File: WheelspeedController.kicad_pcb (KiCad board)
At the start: 4 copper layers, 63.5 x 35.6 mm, 70 parts, among them J1 DEUTSCH DT Inp, J2 DEUTSCH DT Data, J3 DEUTSCH DT Out, J4 Conn_01x02, J6 SWD, SW1 SW_SPDT, SW2 SW_SPDT, U1 LMR51420, U2 AMS1117-3.3, U3 STM32F105RCTx, U4 SN65HVD230, Y1 16MHz

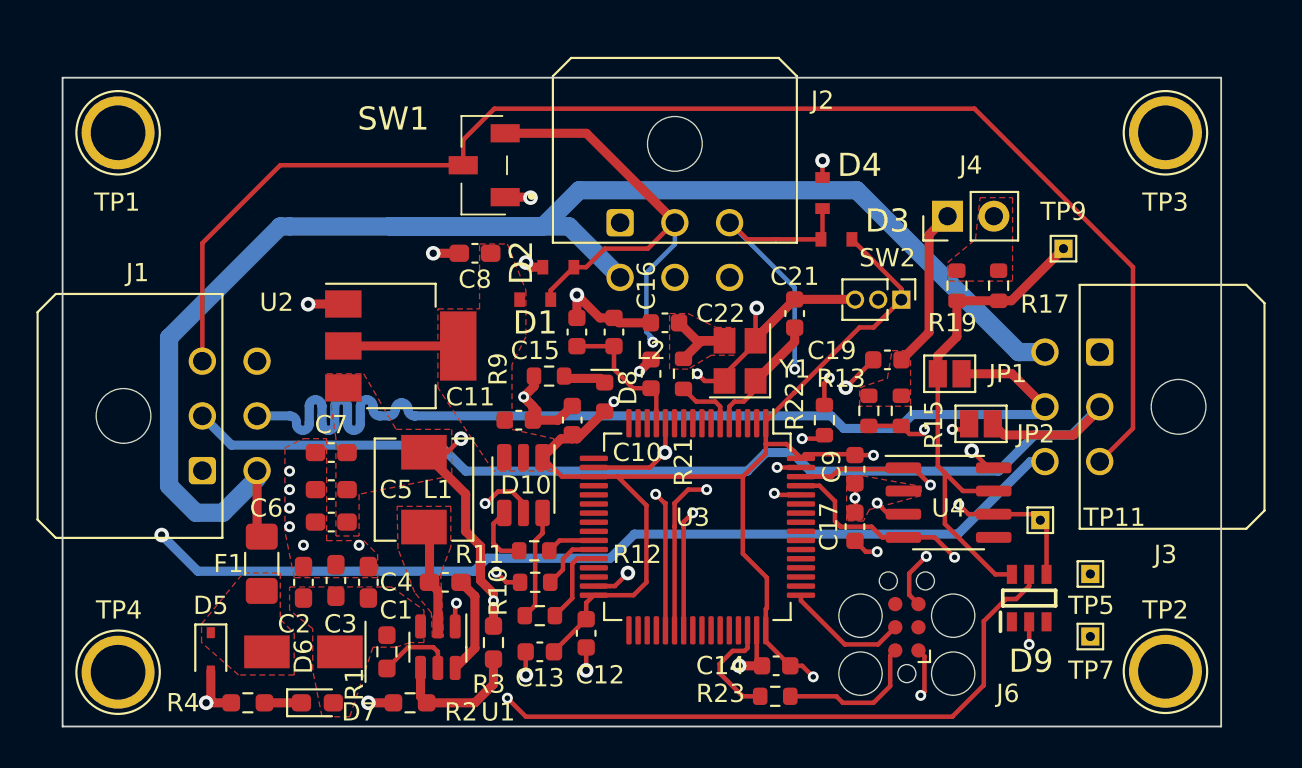
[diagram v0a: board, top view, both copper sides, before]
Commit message: Aligned connectors
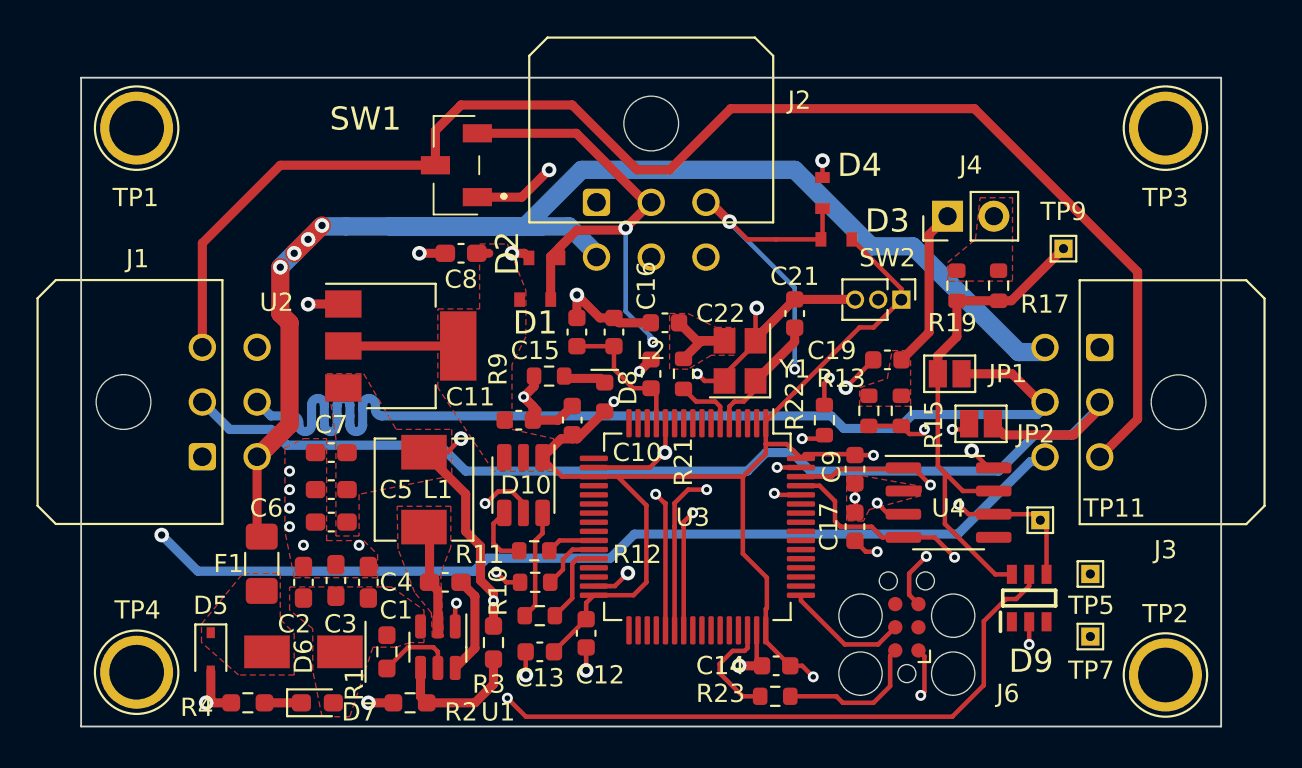
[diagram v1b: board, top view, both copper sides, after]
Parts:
- moved J2 1.71 mm to (87.2, 76.7)
- moved SW1 1.52 mm to (79.5, 74.7)
- moved TP1 1.05 mm to (62.0, 72.6)
- moved TP4 1.02 mm to (62.0, 102.5)
- moved D2 0.92 mm to (84.3, 79.8)
- moved C8 0.76 mm to (79.8, 79.5)
- moved J1 0.76 mm to (65.6, 90.7)
- moved J3 0.25 mm to (114.8, 84.7)
- moved TP3 0.25 mm to (118.4, 72.6)
- moved TP2 0.20 mm to (118.4, 102.6)
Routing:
- net +24V: track 89.3 -> 82.2 mm, vias 0 -> 4
- net /WheelIn1: track 47.2 -> 49.9 mm, vias 3 -> 4
- net /PassThru: track 76.4 -> 78.8 mm
- net /WheelIn2: track 44.5 -> 45.5 mm, vias 2 -> 3
- net +5V: track 69.8 -> 68.9 mm
- net /SHIELD: track 64.9 -> 65.7 mm
- net +3V3: track 94.9 -> 95.6 mm
- net /Extra1: track 21.5 -> 22.0 mm
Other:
- board size 63.5 x 35.6 mm -> 62.5 x 35.6 mm

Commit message: gerbers
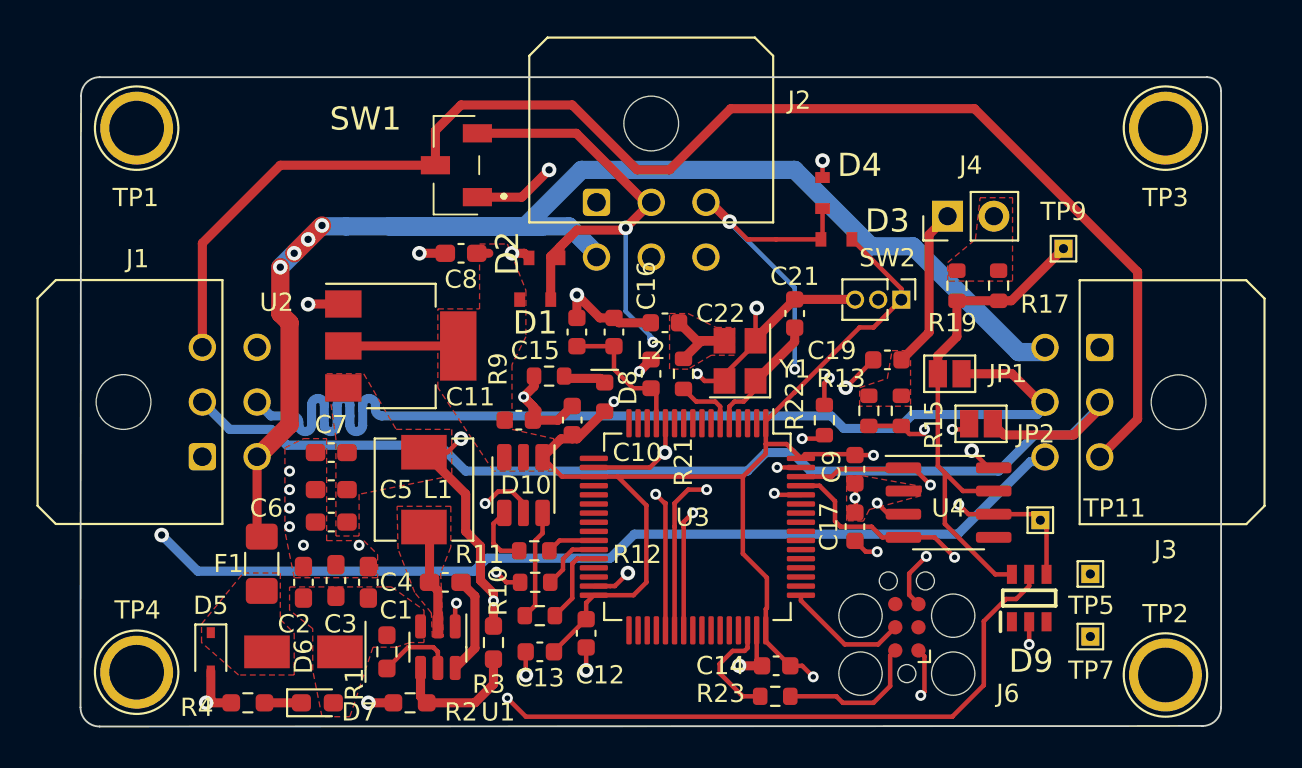
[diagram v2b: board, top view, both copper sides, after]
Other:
- outline, holes or cut-outs redrawn
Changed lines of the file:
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@@
       (layerselection 0x00010fc_ffffffff)
       (disableapertmacros false)
-      (usegerberextensions false)
+      (usegerberextensions true)
       (usegerberattributes true)
       (usegerberadvancedattributes true)
@@
       (plotinvisibletext false)
       (sketchpadsonfab false)
-      (subtractmaskfromsilk false)
+      (subtractmaskfromsilk true)
       (outputformat 1)
       (mirror false)
-      (drillshape 1)
+      (drillshape 0)
       (scaleselection 1)
-      (outputdirectory "")
+      (outputdirectory "Gerbers/")
     )
   )
@@
     (fp_line (start -0.75 0.99) (end 0 0) (layer "F.Fab") (width 0.1))
     (pad "" np_thru_hole circle locked (at 3 -4.32) (size 3 3) (drill 3) (layers *.Cu *.Mask))
-    (pad "1" thru_hole roundrect locked (at 0 0) (size 1.5 1.5) (drill 1.02) (layers *.Cu *.Mask) (roundrect_rratio 0.166667)
+    (pad "1" thru_hole roundrect locked (at 0 0) (size 1.5 1.5) (drill 1.02) (layers *.Cu *.Mask) (roundrect_rratio 0.1666673333)
       (net 1 "GND") (pinfunction "Pin_1") (pintype "passive"))
     (pad "2" thru_hole circle locked (at 3 0) (size 1.5 1.5) (drill 1.02) (layers *.Cu *.Mask)
@@
     (fp_line (start 1.6 0.8) (end -1.6 0.8) (layer "F.Fab") (width 0.1))
     (fp_line (start 1.6 -0.8) (end 1.6 0.8) (layer "F.Fab") (width 0.1))
-    (pad "1" smd roundrect locked (at -1.4875 0 90) (size 1.425 1.75) (layers "F.Cu" "F.Paste" "F.Mask") (roundrect_rratio 0.175439)
+    (pad "1" smd roundrect locked (at -1.4875 0 90) (size 1.425 1.75) (layers "F.Cu" "F.Paste" "F.Mask") (roundrect_rratio 0.1754392982)
       (net 17 "/VRM/DIODE") (pintype "passive"))
-    (pad "2" smd roundrect locked (at 1.4875 0 90) (size 1.425 1.75) (layers "F.Cu" "F.Paste" "F.Mask") (roundrect_rratio 0.175439)
+    (pad "2" smd roundrect locked (at 1.4875 0 90) (size 1.425 1.75) (layers "F.Cu" "F.Paste" "F.Mask") (roundrect_rratio 0.1754392982)
       (net 76 "+24V") (pintype "passive"))
     (model "${KISYS3DMOD}/Fuse.3dshapes/Fuse_1206_3216Metric.wrl"
@@
     (fp_line (start 9.575 -7.92) (end 9.575 0.99) (layer "F.Fab") (width 0.1))
     (pad "" np_thru_hole circle locked (at 3 -4.32 90) (size 3 3) (drill 3) (layers *.Cu *.Mask))
-    (pad "1" thru_hole roundrect locked (at 0 0 90) (size 1.5 1.5) (drill 1.02) (layers *.Cu *.Mask) (roundrect_rratio 0.166667)
+    (pad "1" thru_hole roundrect locked (at 0 0 90) (size 1.5 1.5) (drill 1.02) (layers *.Cu *.Mask) (roundrect_rratio 0.1666673333)
       (net 1 "GND") (pinfunction "Pin_1") (pintype "passive"))
     (pad "2" thru_hole circle locked (at 3 0 90) (size 1.5 1.5) (drill 1.02) (layers *.Cu *.Mask)
@@
     (fp_line (start 9.575 0.99) (end -3.575 0.99) (layer "F.Fab") (width 0.1))
     (pad "" np_thru_hole circle locked (at 3 -4.32 270) (size 3 3) (drill 3) (layers *.Cu *.Mask))
-    (pad "1" thru_hole roundrect locked (at 0 0 270) (size 1.5 1.5) (drill 1.02) (layers *.Cu *.Mask) (roundrect_rratio 0.166667)
+    (pad "1" thru_hole roundrect locked (at 0 0 270) (size 1.5 1.5) (drill 1.02) (layers *.Cu *.Mask) (roundrect_rratio 0.1666673333)
       (net 1 "GND") (pinfunction "Pin_1") (pintype "passive"))
     (pad "2" thru_hole circle locked (at 3 0 270) (size 1.5 1.5) (drill 1.02) (layers *.Cu *.Mask)
@@
       (net 23 "unconnected-(J6-Pad6)") (pinfunction "Pin_6") (pintype "passive+no_connect"))
   )
-  (gr_rect (start 58.933 69.879) (end 121.417 105.439) (layer "Edge.Cuts") (width 0.1) (fill none))
+  (gr_arc (start 121.412 104.394) (mid 121.11442 105.11242) (end 120.396 105.41) (layer "Edge.Cuts") (width 0.1))
+  (gr_line (start 59.944 69.85) (end 120.65 69.85) (layer "Edge.Cuts") (width 0.1))
+  (gr_line (start 121.412 70.612) (end 121.412 104.394) (layer "Edge.Cuts") (width 0.1))
+  (gr_arc (start 120.65 69.85) (mid 121.188815 70.073185) (end 121.412 70.612) (layer "Edge.Cuts") (width 0.1))
+  (gr_arc (start 58.928 70.866) (mid 59.22558 70.14758) (end 59.944 69.85) (layer "Edge.Cuts") (width 0.1))
+  (gr_line (start 120.396 105.41) (end 59.944 105.439) (layer "Edge.Cuts") (width 0.1))
+  (gr_line (start 58.899 104.394) (end 58.928 70.866) (layer "Edge.Cuts") (width 0.1))
+  (gr_arc (start 59.944 105.439) (mid 59.205073 105.132927) (end 58.899 104.394) (layer "Edge.Cuts") (width 0.1))
   (segment (start 90.113 91.243) (end 90.932 90.424) (width 0.25) (layer "F.Cu") (net 1))
   (segment (start 78.8935 79.502) (end 77.47 79.502) (width 0.5) (layer "F.Cu") (net 1))
